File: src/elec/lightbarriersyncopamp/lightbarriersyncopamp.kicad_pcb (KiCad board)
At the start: 2 copper layers, 18.2 x 45 mm, 49 parts, among them J1 Conn_01x03_Pin, Q1 BSS84, Q2 BSS123, Q3 BC850, Q4 BSS123, Q5 BSS123, Q6 BC850, Q7 BSS123, U1 LP2951-3.3_SOIC, U2 TLV9004IDR

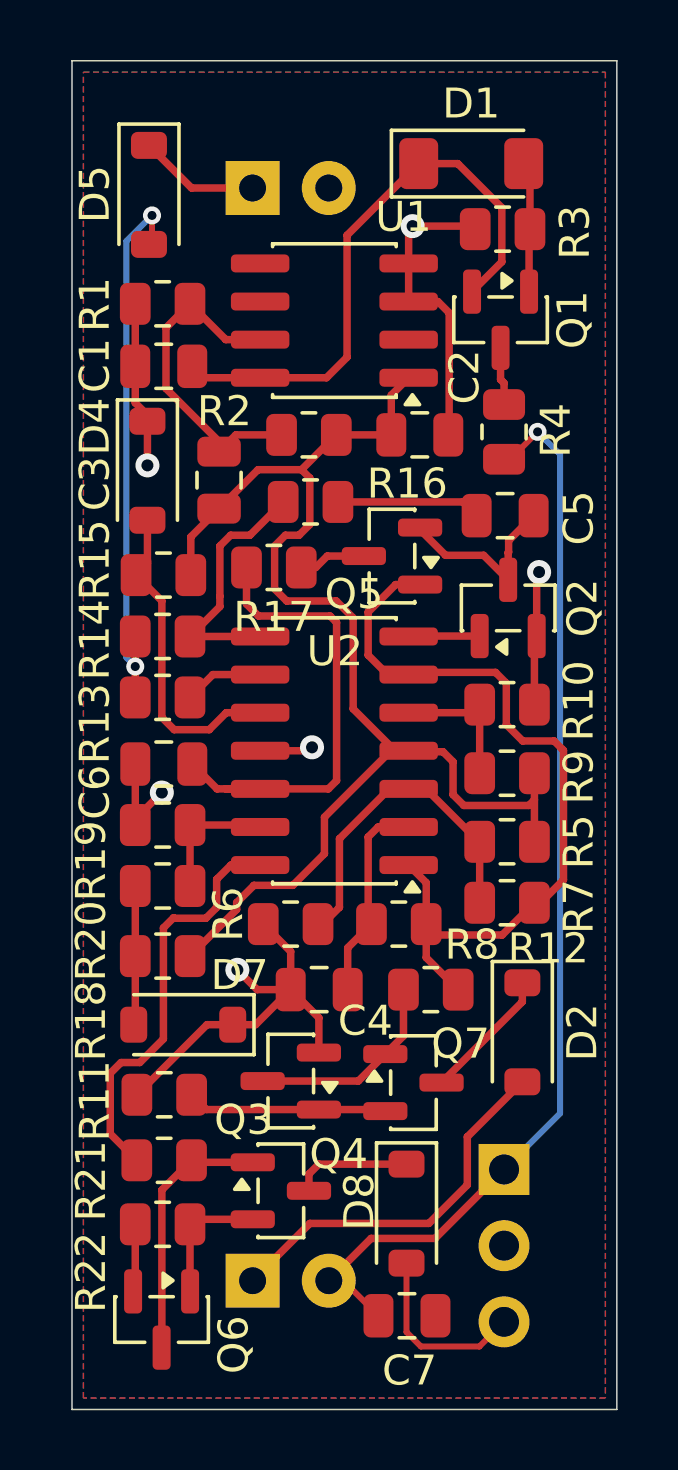
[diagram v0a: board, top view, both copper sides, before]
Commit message: version 0.2 optimized with less components
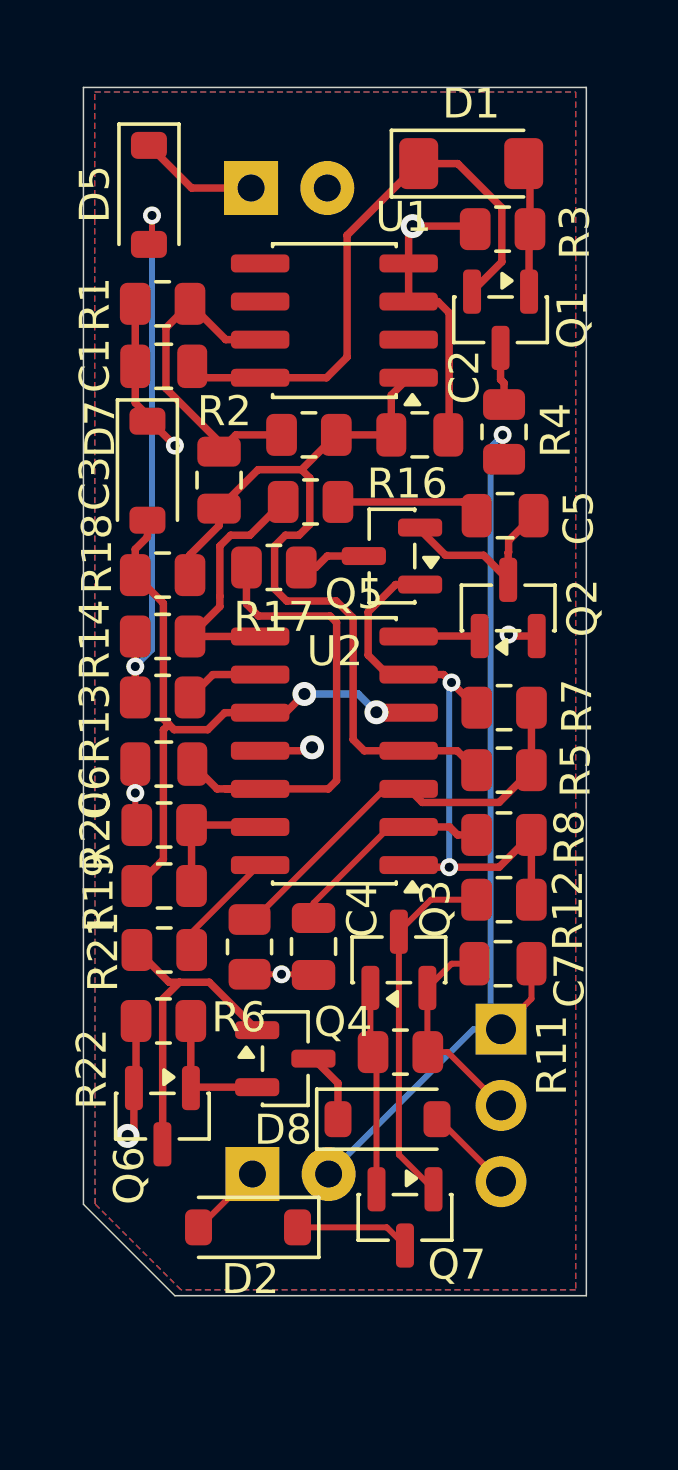
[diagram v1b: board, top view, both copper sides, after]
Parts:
- removed D4: 1N4148W, Diode_SMD:D_SOD-123
- removed R10, R15, R9: 10k, Resistor_SMD:R_0805_2012Metric
- removed the REF** at (111.7, 100.3)
- C5: value 100n -> 1n
- D3: value LD271 -> WP7113F3BT
- D6: value SFH203 -> WP7113PD1BT
- moved D7 18.5 mm to (103.0, 98.1), turned to -90 degrees
- moved R18 12.7 mm to (103.5, 101.6)
- moved C7 12.2 mm to (114.8, 114.6), turned to 180 degrees
- moved D2 11.2 mm to (106.3, 123.3), turned to 180 degrees
- moved REF** 10.7 mm to (109.5, 98.3)
- moved R11 8.00 mm to (111.4, 117.5), turned to 0 degrees
- moved R21 7.01 mm to (103.5, 114.1), turned to 180 degrees
- moved Q6 6.78 mm to (103.5, 119.6)
- moved R22 6.78 mm to (103.5, 116.5)
- moved R7 6.50 mm to (114.9, 106.0), turned to 180 degrees
- moved Q3 5.41 mm to (111.4, 114.4), turned to 90 degrees
- moved J1 4.67 mm to (114.8, 116.7)
- moved R8 4.60 mm to (114.9, 110.3)
- moved Q7 4.50 mm to (111.6, 123.0), turned to -90 degrees
- moved Q4 4.41 mm to (107.6, 117.7)
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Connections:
- U2 pad 10: Net-(D4-A) -> Net-(D7-A)
- U2 pad 5: Net-(U2B-+) -> Net-(D7-A)
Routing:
- net Net-(D7-A): track 4.34 -> 22.1 mm, vias 0 -> 2
- net VDD: track 43.5 -> 28.0 mm
- net Net-(D4-A): track 11.1 -> 0.00 mm
- net Net-(D2-A): track 12.7 -> 2.53 mm
- net Net-(R21-Pad1): track 13.9 -> 3.80 mm
- net GND: track 41.5 -> 33.9 mm, vias 6 -> 7
- net Net-(Q5-G): track 26.8 -> 20.8 mm, vias 0 -> 2
- net VIN: track 36.7 -> 31.3 mm
- net Net-(Q3-C): track 6.86 -> 12.1 mm
- net Net-(U2B-+): track 4.96 -> 0.00 mm
- net Net-(D8-A): track 6.09 -> 3.00 mm
- net Net-(U2A-+): track 11.4 -> 13.9 mm
- net Net-(Q4-G): track 8.72 -> 10.8 mm
- net Net-(D8-K): track 3.95 -> 2.36 mm
- net Net-(D2-K): track 4.44 -> 3.83 mm
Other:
- board size 18.2 x 45 mm -> 16.8 x 40.3 mm
